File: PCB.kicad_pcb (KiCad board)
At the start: 2 copper layers, 70 x 70 mm, 89 parts, among them J1 USB_C_Receptacle_USB2.0_16P, J10 Conn_01x02_Pin, J11 Conn_01x05_Pin, J12 Conn_01x02_Pin, J13 Conn_01x04_Pin, J14 Conn_01x04_Pin, J15 Conn_01x02_Pin, J16 Conn_01x05_Pin, J17 Conn_01x03_Pin, J18 Conn_01x03_Pin, J19 Conn_01x03_Pin, J2 Conn_01x11_Socket, J20 Conn_01x03_Pin, J21 Conn_01x05_Pin, J22 Conn_01x04_Pin, J23 Conn_01x03_Pin, J24 Conn_01x03_Pin, J25 Conn_01x03_Pin, J26 Conn_01x03_Pin, J27 Conn_01x02_Pin, J3 Conn_01x08_Socket, J4 Conn_01x11_Socket, J5 Conn_01x02_Pin, J6 Conn_01x02_Pin, J7 Conn_01x02_Pin, J8 Conn_01x03_Pin, J9 Conn_01x02_Pin, Q1 IRF4905, SW1 SW_Push, SW2 SW_Push, U1 TB6612FNG, U10 MCP23008-xSO, U2 LTC4412xS6, U3 LTC4412xS6, U4 AMS1117-3.3 (UMW), U5 TB6612FNG, U6 ESP32-S3-WROOM-1, U7 TMC2209_SILENTSTEPSTICK, U8 TMC2209_SILENTSTEPSTICK, U9 TMC2209_SILENTSTEPSTICK

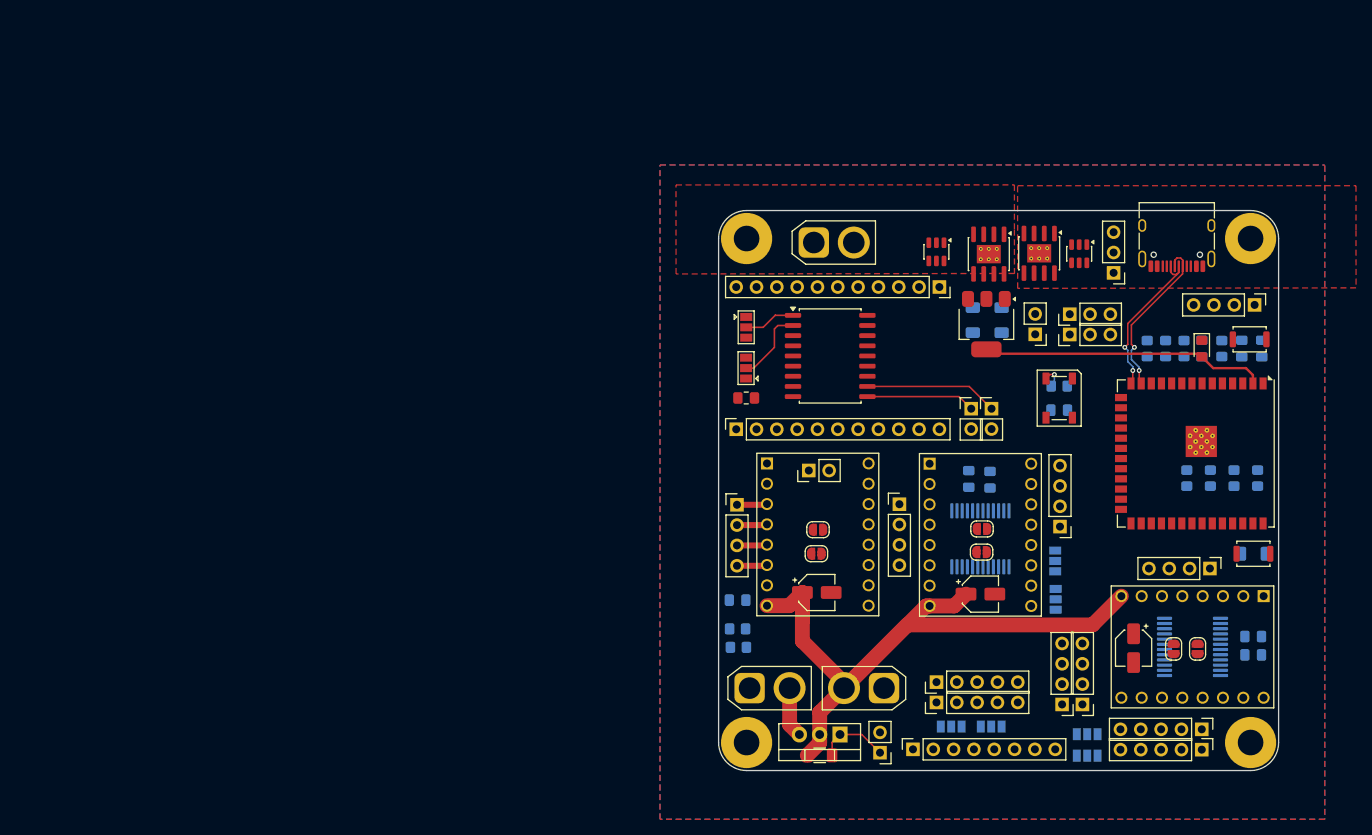
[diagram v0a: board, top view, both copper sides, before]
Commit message: fix BAU + bug
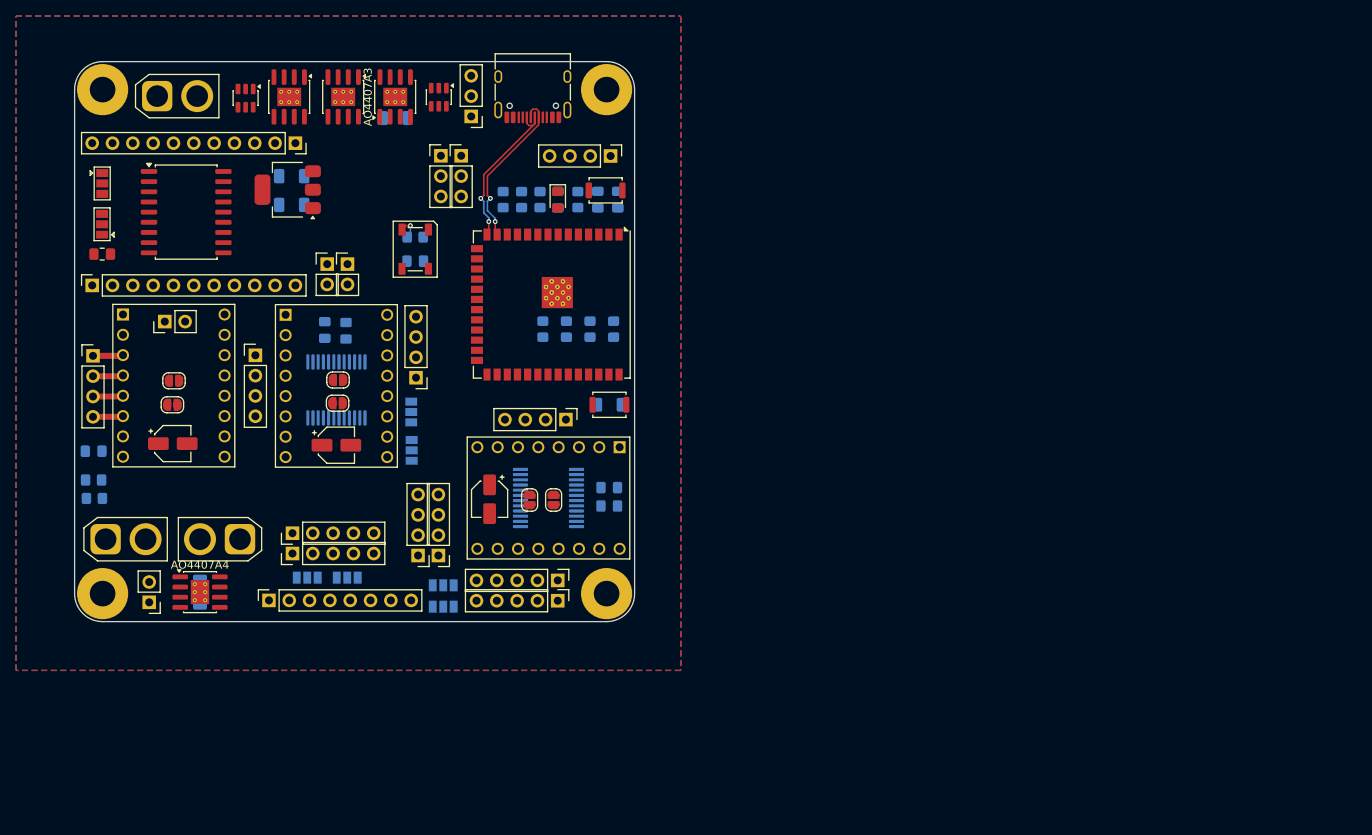
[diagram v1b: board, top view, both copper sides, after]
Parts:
- removed J12: Conn_01x02_Pin, Connector_PinHeader_2.54mm:PinHeader_1x02_P2.54mm_Vertical
- removed Q1: IRF4905, Package_TO_SOT_THT:TO-220-3_Vertical
- added AO4407A3: PMOS, Package_SO:SOIC-8-1EP_3.9x4.9mm_P1.27mm_EP2.29x3mm_ThermalVias, F.Cu at (71.5, 46.1)
- added AO4407A4: PMOS, Package_SO:SOIC-8-1EP_3.9x4.9mm_P1.27mm_EP2.29x3mm_ThermalVias, F.Cu at (47.1, 108.0)
- added R16: 10k, Resistor_SMD:R_1206_3216Metric_Pad1.30x1.75mm_HandSolder, B.Cu at (71.5, 48.8)
- R13: moved to B.Cu
- moved J9 93.3 mm to (40.8, 109.3)
- moved C7 89.9 mm to (58.6, 59.6), turned to 0 degrees
- moved AO4407A2 89.6 mm to (58.2, 46.1)
- moved AO4407A1 89.2 mm to (65.0, 46.1)
- moved U4 88.9 mm to (58.1, 57.7), turned to 180 degrees
- moved U3 88.5 mm to (52.8, 46.2)
- moved C5 87.0 mm to (58.6, 56.0), turned to 0 degrees
- moved J15 84.1 mm to (41.8, 46.0)
- moved J8 82.6 mm to (81.0, 48.5)
- moved AS2 82.6 mm to (74.4, 103.4)
- moved C14 82.6 mm to (83.3, 96.4)
- moved H1 82.6 mm to (97.9, 108.2)
- moved H3 82.6 mm to (97.9, 45.2)
- moved JP1 82.6 mm to (91.3, 96.5)
- moved JP2 82.6 mm to (88.3, 96.5)
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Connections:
- C3 pad 1: VCC_5V_GLOBAL -> 3V3
- C8 pad 1: VCC_5V_GLOBAL -> 3V3
- J1 pad A4: VCC_5V_USB -> VCC_5V_USB_IN
- J1 pad A9: VCC_5V_USB -> VCC_5V_USB_IN
- J1 pad B4: VCC_5V_USB -> VCC_5V_USB_IN
- J1 pad B9: VCC_5V_USB -> VCC_5V_USB_IN
- R13 pad 1: VCC_12V -> VCC_12V_IN
- U1 pad 19: VCC_5V_GLOBAL -> EN1
- U1 pad 20: VCC_5V_GLOBAL -> 3V3
- U5 pad 19: VCC_5V_GLOBAL -> EN2
- U5 pad 20: VCC_5V_GLOBAL -> 3V3
- U7 pad 10: unconnected-(U7-STEP-Pad10) -> M1_IN1
- U7 pad 16: EN2 -> EN1
- U7 pad 9: unconnected-(U7-DIR-Pad9) -> M1_IN2
- U8 pad 10: unconnected-(U8-STEP-Pad10) -> M3_IN1
- U8 pad 9: unconnected-(U8-DIR-Pad9) -> M3_IN2
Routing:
- net VCC_12V: track 92.6 -> 0.00 mm
- net 3V3: track 35.7 -> 0.00 mm
- net LAUNCHPULL: track 16.7 -> 0.00 mm
- net TEAM_BTN: track 13.6 -> 0.00 mm
- net Net-(J18-Pin_2): track 9.43 -> 0.00 mm
- net BAU+: track 8.95 -> 0.00 mm
- net Net-(J17-Pin_2): track 6.47 -> 0.00 mm
- net VCC_12V_IN: track 6.31 -> 0.00 mm
- removed copper zone on F.Cu, net VCC_5V_BUCK
- removed copper zone on F.Cu, net VCC_5V_USB
